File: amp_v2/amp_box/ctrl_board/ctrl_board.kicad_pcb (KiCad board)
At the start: 2 copper layers, 45.1 x 70 mm, 36 parts, among them IC1 L293D, J1 Atmega328, U1 7805

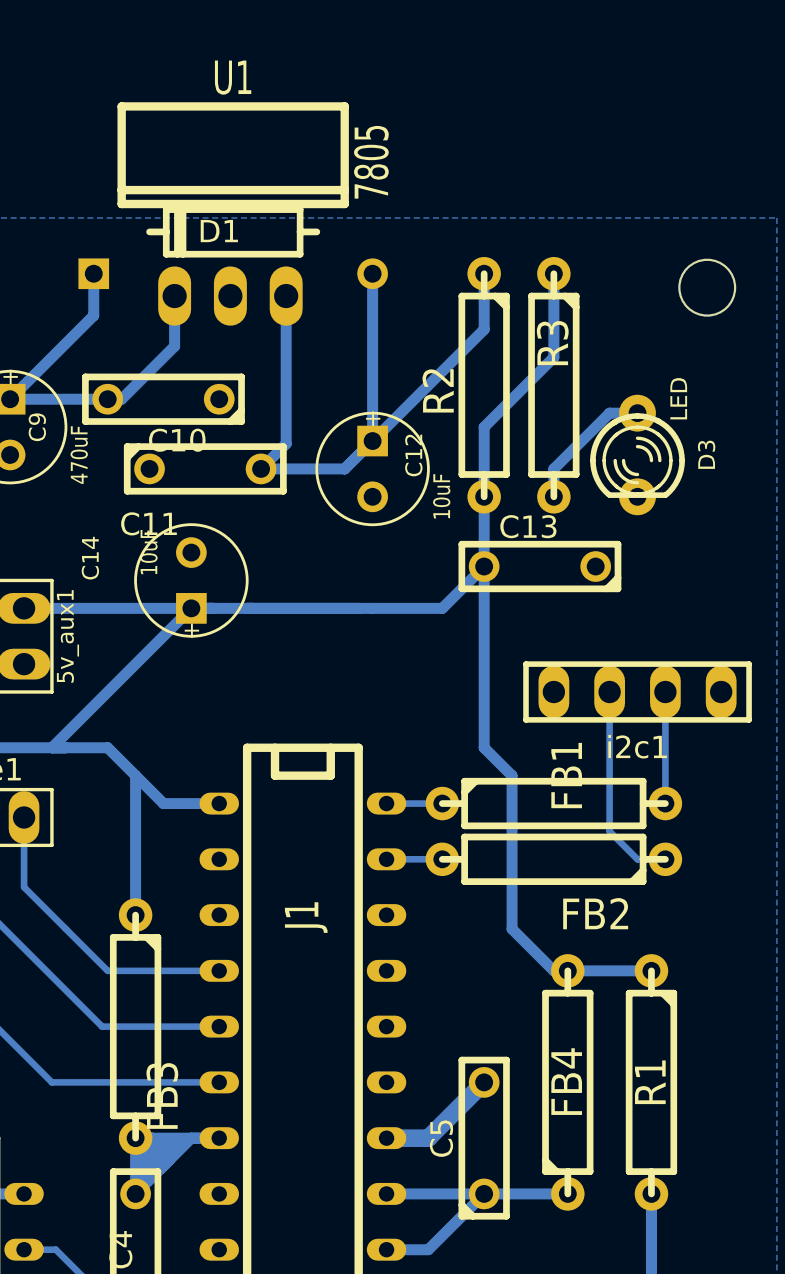
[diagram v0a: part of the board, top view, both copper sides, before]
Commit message: updates
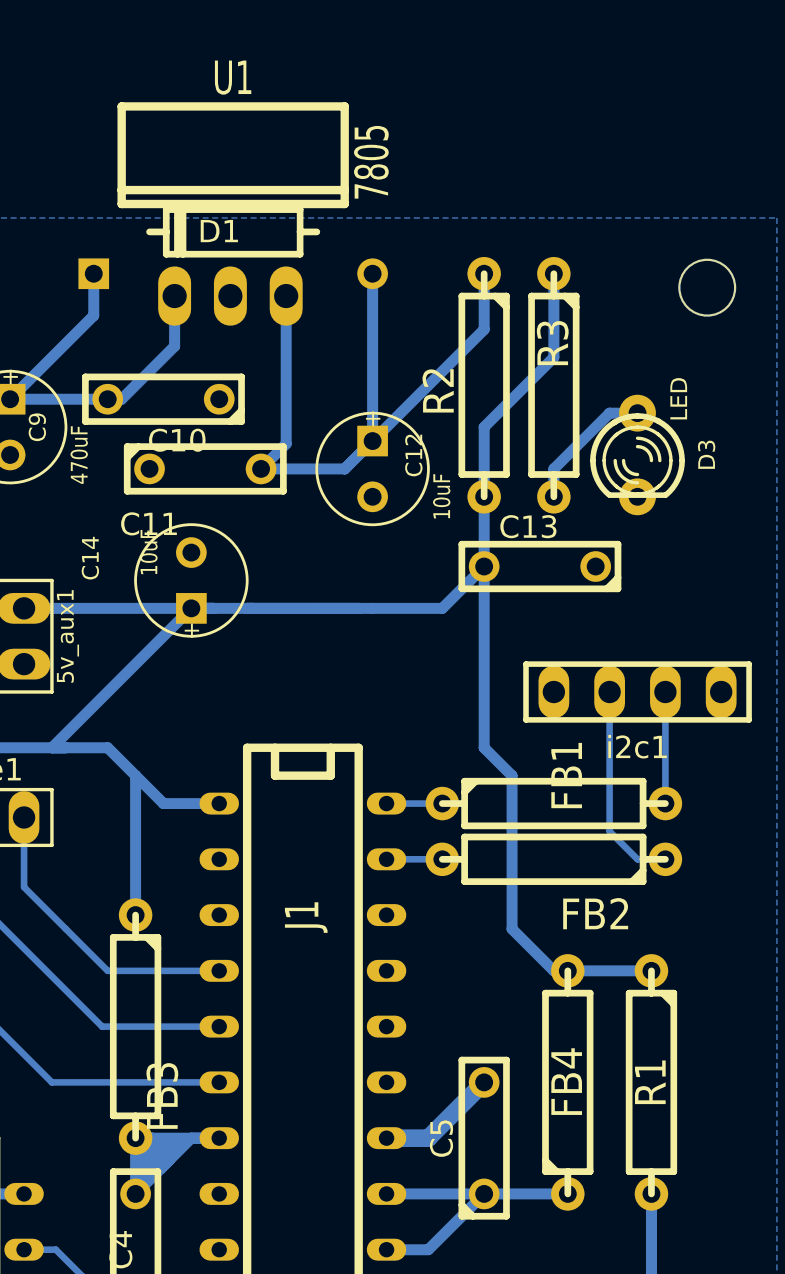
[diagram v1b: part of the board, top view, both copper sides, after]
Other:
- net class Default removed
- net class pwr removed
